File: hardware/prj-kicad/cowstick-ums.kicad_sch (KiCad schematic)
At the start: 27 parts, among them J1 CONN_USB-A, U1 STM32G0KxT, U2 LM3671, U3 W25QxxVSN, U4 W25QxxVSN, U5 W25NxxVZE, U90 AZ2210, X1 32,768k

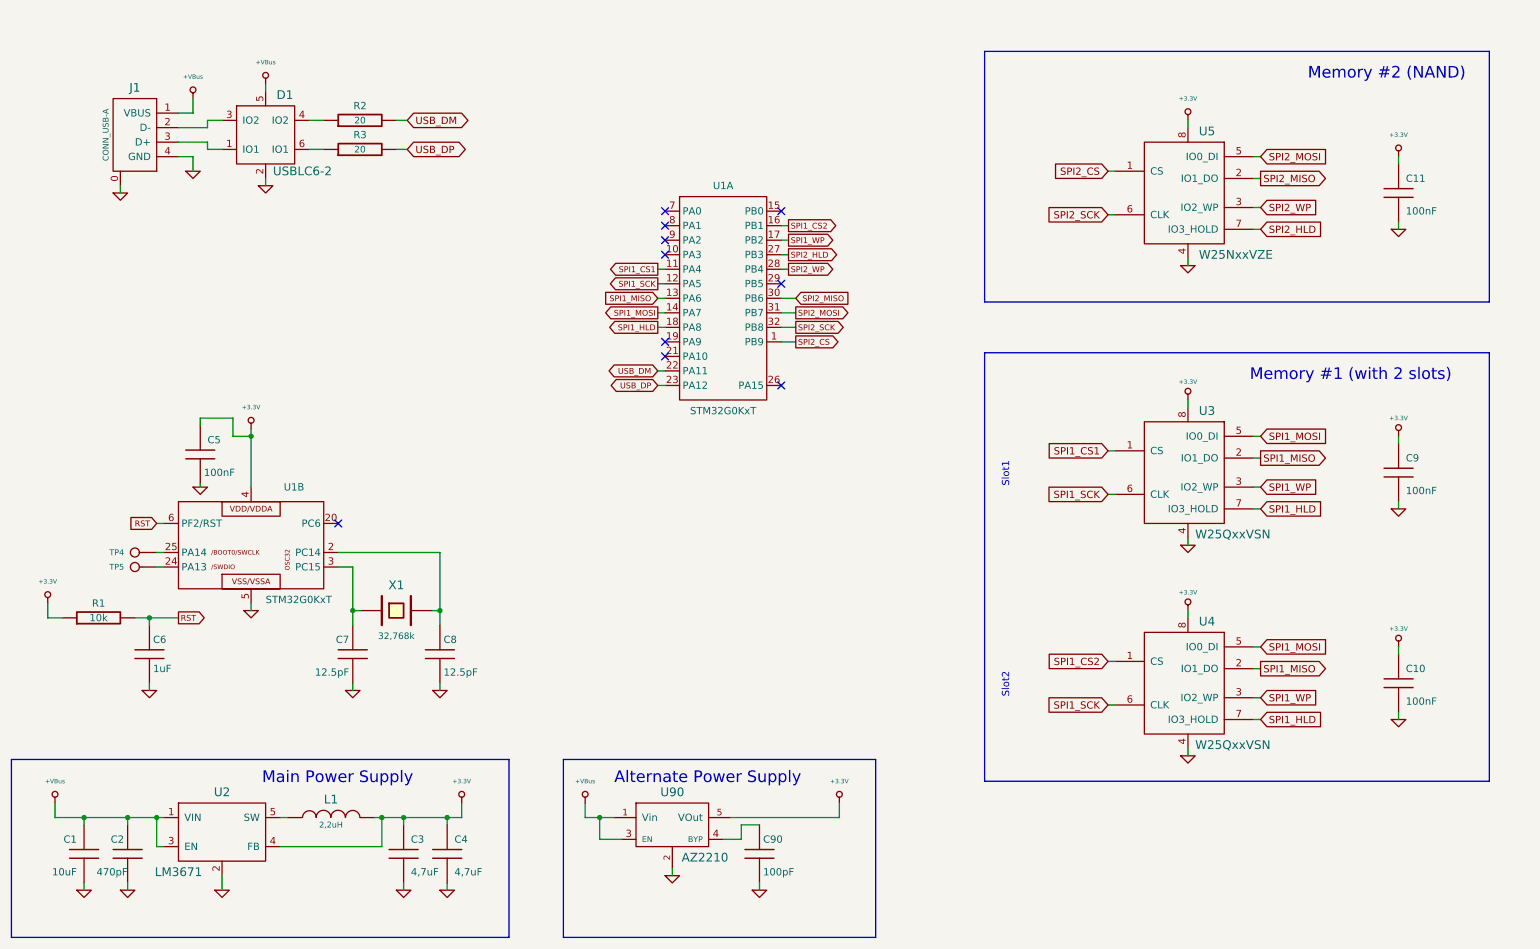
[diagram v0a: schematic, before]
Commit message: Hardware: Finish and cleanup pcb r1 and create production files
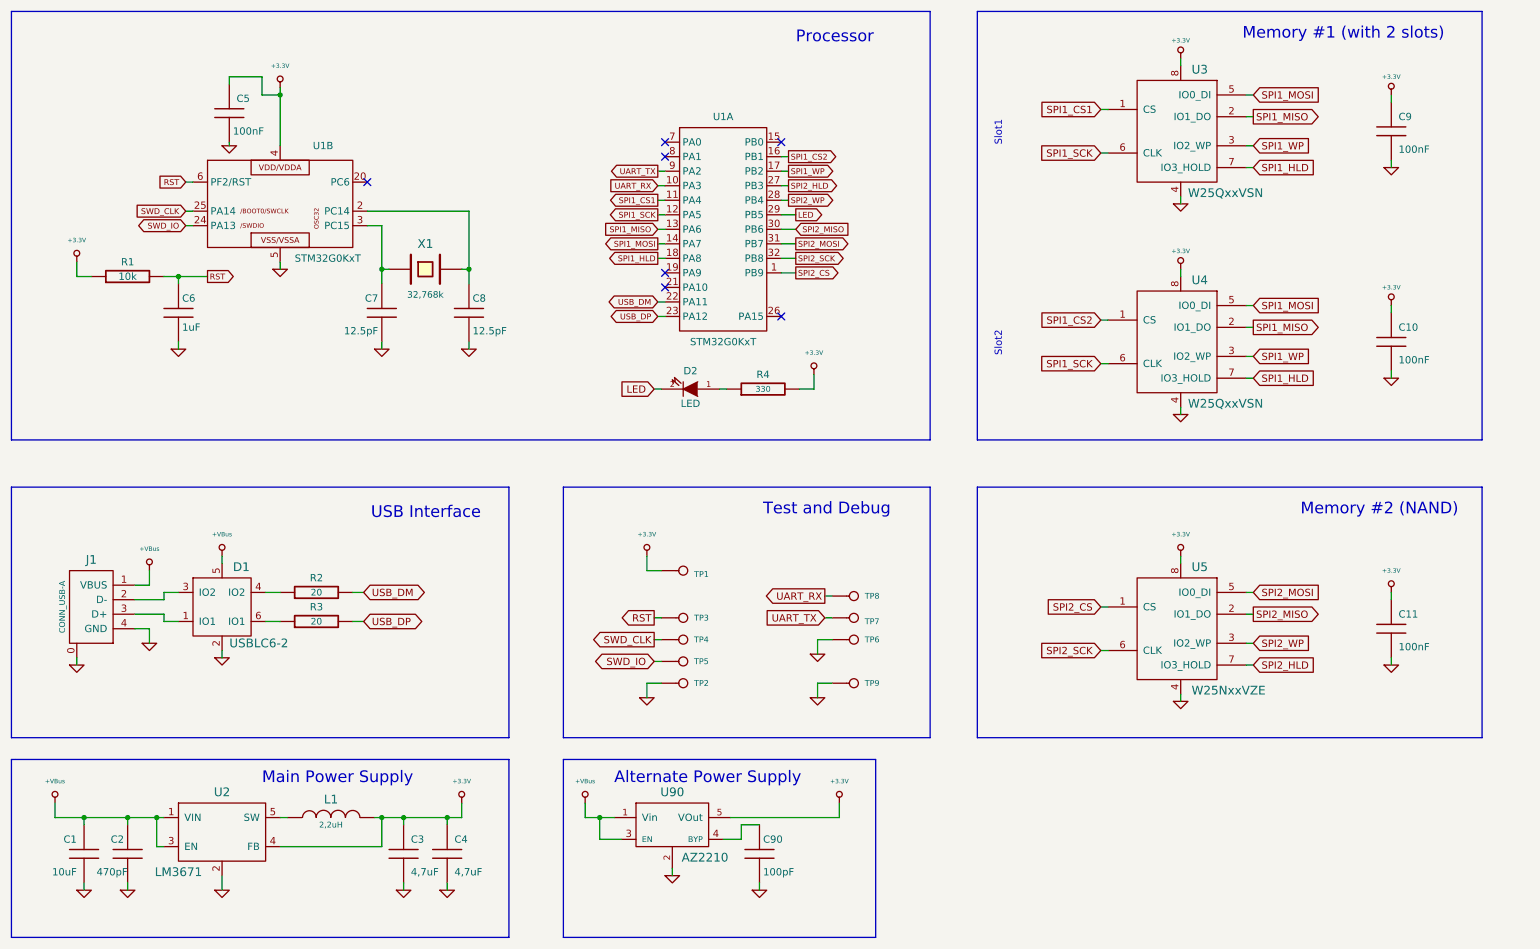
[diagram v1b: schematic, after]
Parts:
- added D2: LED, cowstick-ums:C_0805, symbol cowstick-ums:LED
- added R4: 330, cowstick-ums:R_0603, symbol cowstick-ums:R
- added TP1, TP2, TP3: CONN_1, cowstick-ums:TP_SMD, symbol cowstick-ums:CONN_1
- added TP6, TP7, TP8, TP9: CONN_1, cowstick-ums:TP_PIN, symbol cowstick-ums:CONN_1
- TP4, TP5: footprint (none) -> cowstick-ums:TP_SMD
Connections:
- net +3.3V: now also R4.2, TP1.1
- net GND: now also TP2.1, TP6.1, TP9.1
- net RST: now also TP3.1
- net SWD_IO: now reaches TP5.1, U1.24 (PA13)
- net SWD_CLK: now reaches TP4.1, U1.25 (PA14)
- net UART_RX: now reaches U1.10 (PA3)
- net UART_RX: now also TP8.1
- net LED: now reaches U1.29 (PB5)
- net LED: now also D2.2 (K)
- net UART_TX: now reaches U1.9 (PA2)
- net UART_TX: now also TP7.1
- new net: D2.1 (A), R4.1
- no-connect marks 10 -> 7
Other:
- note added: "Processor"
- note added: "Test and Debug"
- note added: "USB Interface"
- moved on the sheet: C10, C11, C5, C6, C7, C8, C9, D1, J1, R1, R2, R3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
